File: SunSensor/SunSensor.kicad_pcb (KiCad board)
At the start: 2 copper layers, 92.9 x 34.7 mm, 19 parts, among them U1 AD7291BCPZ, U2 FEATHER_M0_BASIC_PROTO

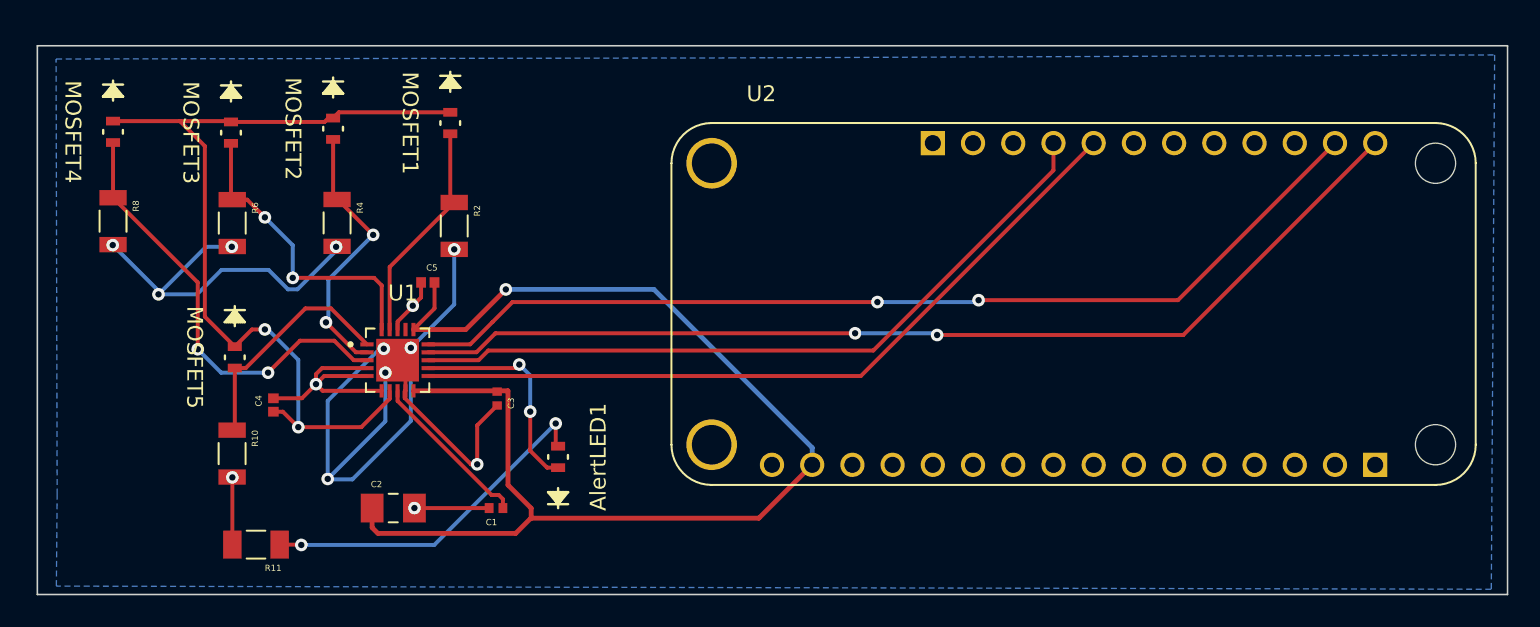
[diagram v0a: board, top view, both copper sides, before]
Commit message: Finish Routing
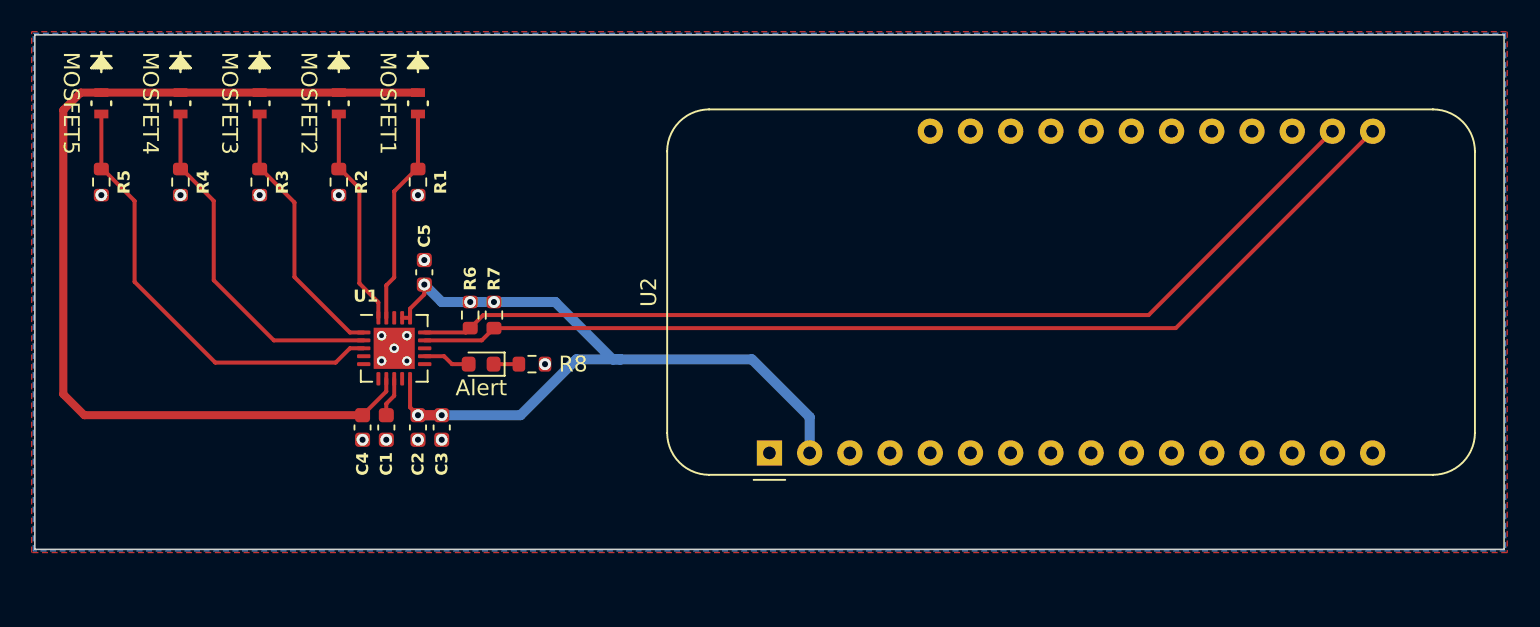
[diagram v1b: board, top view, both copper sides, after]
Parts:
- added R6: 10K, Resistor_SMD:R_0603_1608Metric, F.Cu at (127.3, 99.1)
- added R7: 10K, Resistor_SMD:R_0603_1608Metric, F.Cu at (128.8, 99.1)
- Alert: renamed from AlertLED1; footprint sunsensor:LED_77&slash_TR8_EVE -> LED_SMD:LED_0603_1608Metric
- C1: value 1 µF -> 1uF; footprint sunsensor:CAPC1005X60N -> Capacitor_SMD:C_0603_1608Metric
- C2: value 100 µF -> 10uF; footprint sunsensor:CAPC3216X190N -> Capacitor_SMD:C_0603_1608Metric
- C3: value 100 nF -> 0.1uF; footprint sunsensor:CAPC1005X55N -> Capacitor_SMD:C_0603_1608Metric
- C4: value 10 µF -> 10uF; footprint sunsensor:CAPC1005X71N -> Capacitor_SMD:C_0603_1608Metric
- C5: value 10 µF -> 1uF; footprint sunsensor:CAPC1005X71N -> Capacitor_SMD:C_0603_1608Metric
- R1: renamed from R2; value 50k_Ohms -> 50K; footprint sunsensor:RESC3116X65N -> Resistor_SMD:R_0603_1608Metric
- R2: renamed from R6; value 50k_Ohms -> 50K; footprint sunsensor:RESC3116X65N -> Resistor_SMD:R_0603_1608Metric
- R3: renamed from R10; value 50k_Ohms -> 50K; footprint sunsensor:RESC3116X65N -> Resistor_SMD:R_0603_1608Metric
- R4: value 50k_Ohms -> 50K; footprint sunsensor:RESC3116X65N -> Resistor_SMD:R_0603_1608Metric
- R5: renamed from R8; value 50k_Ohms -> 50K; footprint sunsensor:RESC3116X65N -> Resistor_SMD:R_0603_1608Metric
- R8: renamed from R11; value 1k_ohms -> 1K; footprint sunsensor:RESC3216X75N -> Resistor_SMD:R_0603_1608Metric
- U1: footprint sunsensor:QFN50P400X400X100-21N -> Package_DFN_QFN:QFN-20-1EP_4x4mm_P0.5mm_EP2.6x2.6mm
- U2: footprint sunsensor:MODULE_FEATHER_M0_BASIC_PROTO -> Module:Adafruit_Feather
- moved U2 21.4 mm to (146.2, 107.8), turned to 90 degrees
- moved R8 20.8 mm to (131.2, 102.2), turned to 0 degrees
- moved R3 17.2 mm to (114.0, 90.7)
- moved MOSFET3 16.1 mm to (114.0, 85.7)
- moved R4 10.2 mm to (109.0, 90.7)
- moved MOSFET4 9.77 mm to (109.0, 85.7)
- moved C1 8.60 mm to (122.0, 106.2), turned to -90 degrees
- moved Alert 7.61 mm to (128.0, 102.2), turned to 180 degrees
- moved R2 7.21 mm to (119.0, 90.7)
- moved MOSFET2 7.06 mm to (119.0, 85.7)
- moved C4 5.81 mm to (120.5, 106.2), turned to -90 degrees
- moved C2 5.32 mm to (124.0, 106.2), turned to -90 degrees
- moved C3 3.95 mm to (125.5, 106.2)
- moved R1 3.59 mm to (124.0, 90.7)
- moved R5 2.58 mm to (104.0, 90.7)
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- renumbered MOSFET3 to MOSFET2, MOSFET5 to MOSFET3, MOSFET2 to MOSFET4, MOSFET4 to MOSFET5
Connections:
- Alert pad 1: Net-(AlertLED1-Pad1) -> Net-(AlertLED1-K)
- Alert pad 2: /LEDOUT -> Net-(AlertLED1-A)
- C1 pad 2: GNDREF -> GND
- C2 pad 2: GNDREF -> GND
- C3 pad 2: GNDREF -> GND
- C4 pad 2: GNDREF -> GND
- C5 pad 1: GNDREF -> GND
- R1 pad 2: GNDREF -> GND
- R2 pad 2: GNDREF -> GND
- R3 pad 2: GNDREF -> GND
- R4 pad 2: GNDREF -> GND
- R5 pad 2: GNDREF -> GND
- R8 pad 1: /LEDOUT -> Net-(AlertLED1-K)
- R8 pad 2: GNDREF -> GND
- U1 pad 11: /AS0 -> GND
- U1 pad 12: Net-(AlertLED1-Pad1) -> Net-(AlertLED1-A)
- U1 pad 13: /AS1 -> GND
- U1 pad 17: unconnected-(U1-Pad17) -> +3V3
- U1 pad 18: GNDREF -> GND
- U1 pad 21: GNDREF -> GND
- U1 pad 4: GNDREF -> GND
- U1 pad 5: GNDREF -> GND
- U1 pad 6: GNDREF -> GND
- U1 pad 9: GNDREF -> GND
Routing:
- net GNDREF: track 100.1 -> 0.00 mm, vias 14 -> 0
- net /AS0: track 48.1 -> 0.00 mm
- net /AS1: track 46.2 -> 0.00 mm
- net +3V3: track 80.5 -> 51.3 mm, vias 1 -> 5
- net /LEDOUT: track 22.1 -> 0.00 mm, vias 2 -> 0
- net Net-(AlertLED1-Pad1): track 13.8 -> 0.00 mm, vias 2 -> 0
- net Net-(U1-DCAP): track 10.4 -> 2.51 mm
- net /V_ref: track 55.8 -> 63.2 mm, vias 2 -> 0
- net /Vin2: track 19.3 -> 13.9 mm, vias 2 -> 0
- net /Vin4: track 17.2 -> 22.4 mm, vias 2 -> 0
- net Net-(AlertLED1-A): track 0.00 -> 2.98 mm
- net /Vin3: track 14.8 -> 17.0 mm
- net Net-(AlertLED1-K): track 0.00 -> 1.60 mm
- net /Vin5: track 27.9 -> 28.4 mm, vias 2 -> 0
- net /SCL_chip: track 62.5 -> 62.6 mm, vias 2 -> 0
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- added copper zone on B.Cu, net GND
- added copper zone on F.Cu, net GND
- removed copper zone on B.Cu, net GNDREF
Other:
- board size 92.9 x 34.7 mm -> 92.8 x 32.5 mm
